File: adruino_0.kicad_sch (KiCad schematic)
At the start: 21 parts, among them J1 Conn_01x04_Male, J10 Conn_01x04_Male, J11 Conn_02x02_Odd_Even, J12 Conn_01x02_Male, J13 Conn_02x14_Odd_Even, J14 Conn_02x14_Odd_Even, J15 Conn_01x04_Male, J16 Conn_02x02_Odd_Even, J2 Conn_01x04_Male, J3 Conn_01x04_Male, J4 Conn_01x04_Male, J5 Conn_01x04_Male, J6 Conn_02x02_Odd_Even, J7 Conn_02x02_Odd_Even, J8 Conn_02x02_Odd_Even, J9 Conn_02x02_Odd_Even, U1 W25Q32JVSS

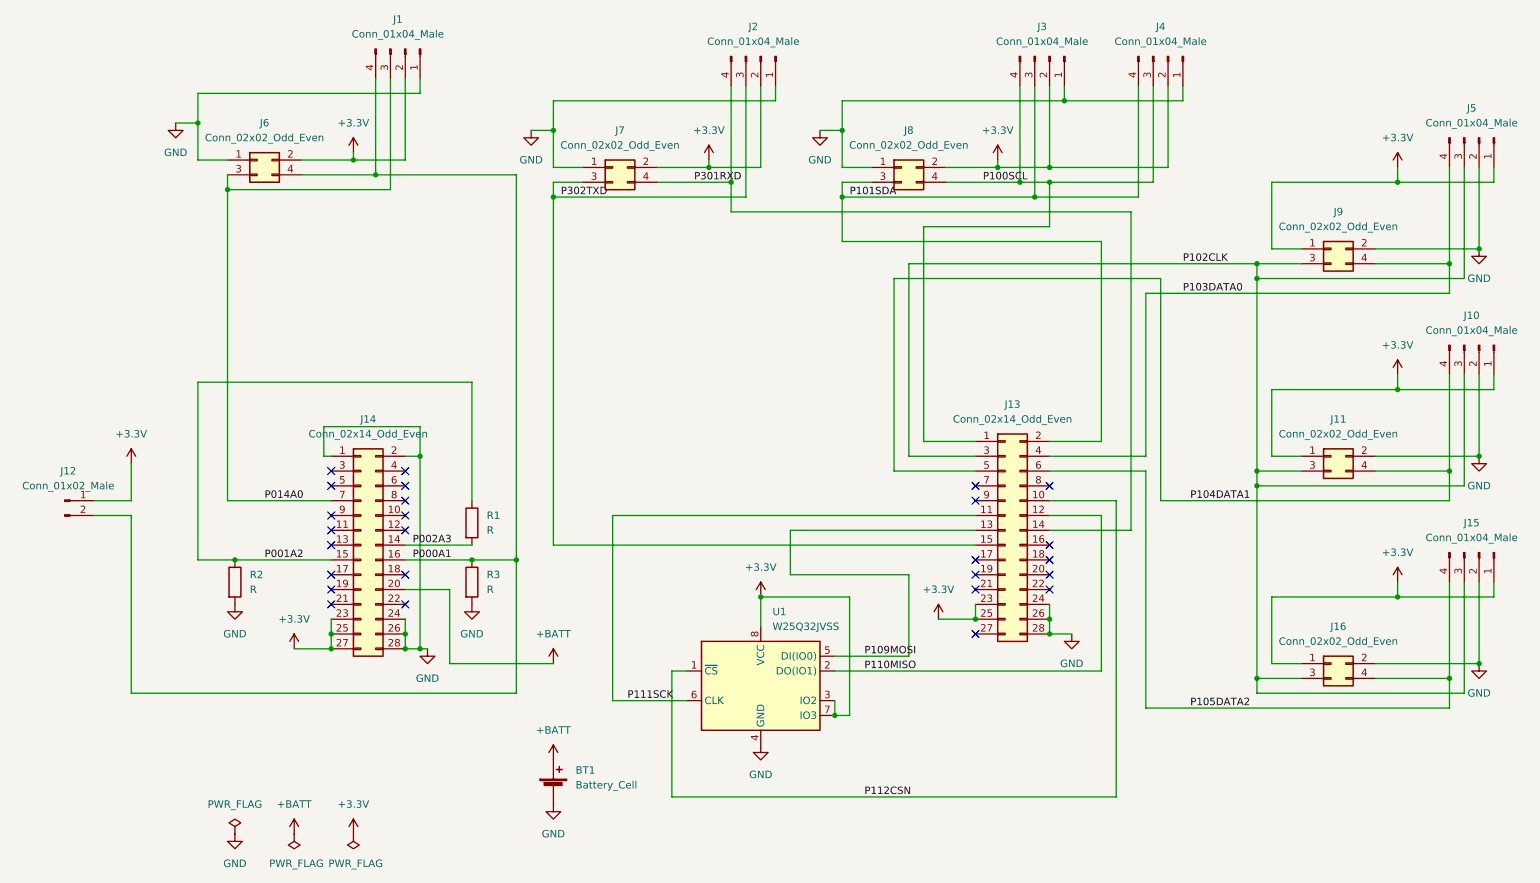
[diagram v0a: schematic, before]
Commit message: 基板更新
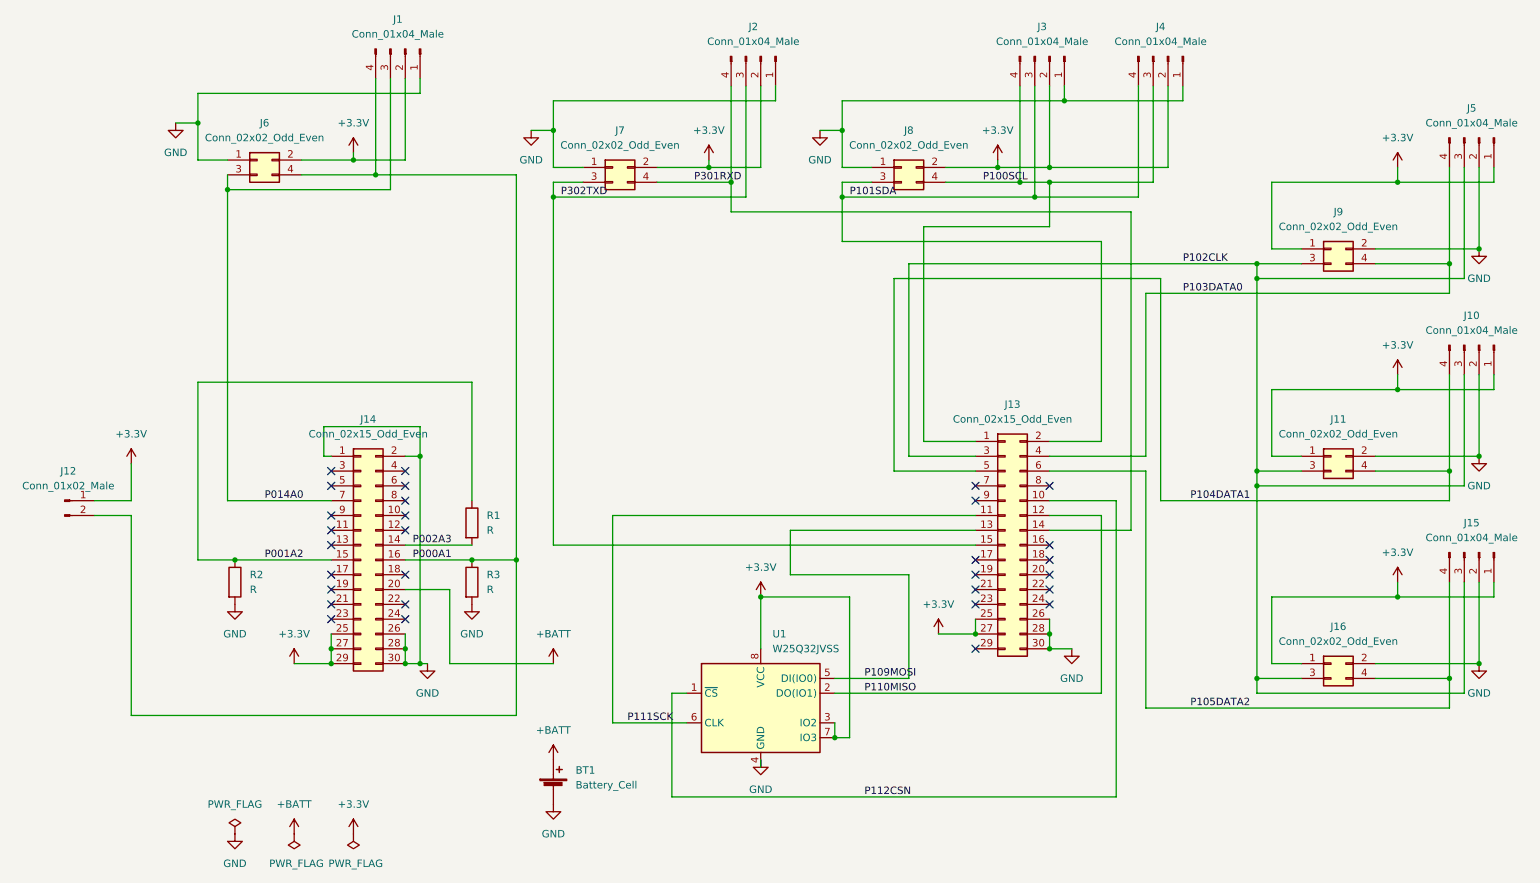
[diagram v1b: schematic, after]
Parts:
- removed J13, J14: Conn_02x14_Odd_Even, Connector_PinSocket_2.54mm:PinSocket_2x14_P2.54mm_Vertical, symbol Connector_Generic:Conn_02x14_Odd_Even
- added J13, J14: Conn_02x15_Odd_Even, Connector_PinHeader_2.54mm:PinHeader_2x15_P2.54mm_Vertical, symbol Connector_Generic:Conn_02x15_Odd_Even
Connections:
- net +3.3V: now also J13.25 (Pin_25), J13.27 (Pin_27), J14.25 (Pin_25), J14.27 (Pin_27), J14.29 (Pin_29)
- net +BATT: now also J14.20 (Pin_20)
- net GND: now also J13.26 (Pin_26), J13.28 (Pin_28), J13.30 (Pin_30), J14.1 (Pin_1), J14.2 (Pin_2), J14.26 (Pin_26), J14.28 (Pin_28), J14.30 (Pin_30)
- net P000A1: now also J14.16 (Pin_16)
- net P001A2: now also J14.15 (Pin_15)
- net P002A3: now also J14.14 (Pin_14)
- net P014A0: now also J14.7 (Pin_7)
- net P100SCL: now also J13.1 (Pin_1)
- net P101SDA: now also J13.2 (Pin_2)
- net P102CLK: now also J13.3 (Pin_3)
- net P103DATA0: now also J13.4 (Pin_4)
- net P104DATA1: now also J13.5 (Pin_5)
- net P105DATA2: now also J13.6 (Pin_6)
- net P109MOSI: now also J13.13 (Pin_13)
- net P110MISO: now also J13.12 (Pin_12)
- net P111SCK: now also J13.11 (Pin_11)
- net P112CSN: now also J13.10 (Pin_10)
- net P301RXD: now also J13.14 (Pin_14)
- net P302TXD: now also J13.15 (Pin_15)
- no-connect marks 26 -> 30
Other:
- moved on the sheet: U1
